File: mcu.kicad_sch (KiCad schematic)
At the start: 9 parts, among them SW1 Push_Button, SW2 Push_Button, U2 ESP32-S3-WROOM-1

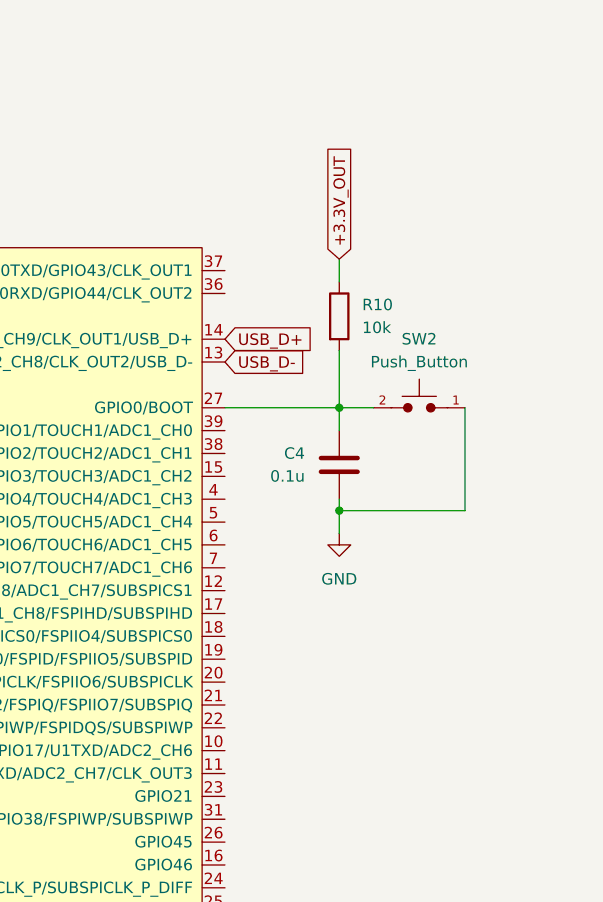
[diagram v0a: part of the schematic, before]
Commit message: Small ammendments
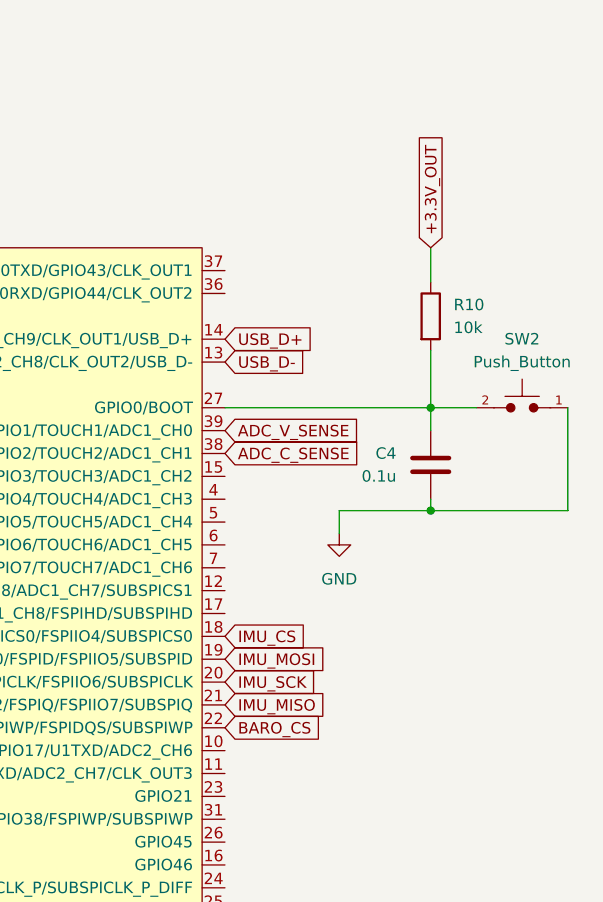
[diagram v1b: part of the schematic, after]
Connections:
- net IMU_CS: now reaches U2.18 (GPIO10/TOUCH10/ADC1_CH9/FSPICS0/FSPIIO4/SUBSPICS0)
- net IMU_MOSI: now reaches U2.19 (GPIO11/TOUCH11/ADC2_CH0/FSPID/FSPIIO5/SUBSPID)
- net IMU_SCK: now reaches U2.20 (GPIO12/TOUCH12/ADC2_CH1/FSPICLK/FSPIIO6/SUBSPICLK)
- net IMU_MISO: now reaches U2.21 (GPIO13/TOUCH13/ADC2_CH2/FSPIQ/FSPIIO7/SUBSPIQ)
- net BARO_CS: now reaches U2.22 (GPIO14/TOUCH14/ADC2_CH3/FSPIWP/FSPIDQS/SUBSPIWP)
- net ADC_C_SENSE: now reaches U2.38 (GPIO2/TOUCH2/ADC1_CH1)
- net ADC_V_SENSE: now reaches U2.39 (GPIO1/TOUCH1/ADC1_CH0)
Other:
- moved on the sheet: C4, R10, SW2
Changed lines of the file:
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@@
 	(paper "A4")
+	(junction
+		(at 156.21 67.31)
+		(diameter 0)
+		(color 0 0 0 0)
+	)
 	(junction
 		(at 76.2 25.4)
@@
 	)
 	(junction
-		(at 146.05 78.74)
+		(at 156.21 78.74)
 		(diameter 0)
 		(color 0 0 0 0)
@@
 	)
 	(junction
-		(at 146.05 67.31)
-		(diameter 0)
-		(color 0 0 0 0)
-	)
-	(junction
 		(at 68.58 36.83)
 		(diameter 0)
@@
 	(wire
 		(pts
+			(xy 146.05 78.74) (xy 146.05 81.28)
+		)
+		(stroke
+			(width 0)
+			(type default)
+		)
+	)
+	(wire
+		(pts
 			(xy 76.2 25.4) (xy 87.63 25.4)
 		)
@@
 	(wire
 		(pts
-			(xy 146.05 67.31) (xy 149.86 67.31)
+			(xy 156.21 67.31) (xy 161.29 67.31)
 		)
 		(stroke
@@
 	(wire
 		(pts
-			(xy 160.02 67.31) (xy 160.02 78.74)
+			(xy 171.45 67.31) (xy 171.45 78.74)
 		)
 		(stroke
@@
 	(wire
 		(pts
-			(xy 146.05 78.74) (xy 160.02 78.74)
+			(xy 146.05 78.74) (xy 156.21 78.74)
 		)
 		(stroke
@@
 	(wire
 		(pts
-			(xy 146.05 67.31) (xy 146.05 69.85)
+			(xy 156.21 67.31) (xy 156.21 69.85)
 		)
 		(stroke
@@
 	(wire
 		(pts
-			(xy 133.35 67.31) (xy 146.05 67.31)
+			(xy 133.35 67.31) (xy 156.21 67.31)
 		)
 		(stroke
@@
 	(wire
 		(pts
+			(xy 156.21 49.53) (xy 156.21 53.34)
+		)
+		(stroke
+			(width 0)
+			(type default)
+		)
+	)
+	(wire
+		(pts
 			(xy 33.02 49.53) (xy 33.02 54.61)
 		)
@@
 	(wire
 		(pts
-			(xy 146.05 50.8) (xy 146.05 53.34)
+			(xy 156.21 78.74) (xy 171.45 78.74)
 		)
 		(stroke
@@
 	(wire
 		(pts
-			(xy 146.05 60.96) (xy 146.05 67.31)
-		)
-		(stroke
-			(width 0)
-			(type default)
-		)
-	)
-	(wire
-		(pts
-			(xy 146.05 77.47) (xy 146.05 81.28)
-		)
-		(stroke
-			(width 0)
-			(type default)
+			(xy 156.21 60.96) (xy 156.21 67.31)
+		)
+		(stroke
+			(width 0)
+			(type default)
+		)
+	)
+	(wire
+		(pts
+			(xy 156.21 77.47) (xy 156.21 78.74)
+		)
+		(stroke
+			(width 0)
+			(type default)
+		)
+	)
+	(global_label "IMU_MOSI"
+		(shape input)
+		(at 133.35 95.25 0)
+		(fields_autoplaced yes)
+		(effects
+			(font
+				(size 1.27 1.27)
+			)
+			(justify left)
+		)
+		(property "Intersheetrefs" "${INTERSHEET_REFS}"
+			(at 145.2857 95.25 0)
+			(hide yes)
+			(show_name no)
+			(do_not_autoplace no)
+			(effects
+				(font
+					(size 1.27 1.27)
+				)
+				(justify left)
+			)
+		)
+	)
+	(global_label "IMU_CS"
+		(shape input)
+		(at 133.35 92.71 0)
+		(fields_autoplaced yes)
+		(effects
+			(font
+				(size 1.27 1.27)
+			)
+			(justify left)
+		)
+		(property "Intersheetrefs" "${INTERSHEET_REFS}"
+			(at 143.169 92.71 0)
+			(hide yes)
+			(show_name no)
+			(do_not_autoplace no)
+			(effects
+				(font
+					(size 1.27 1.27)
+				)
+				(justify left)
+			)
+		)
+	)
+	(global_label "ADC_C_SENSE"
+		(shape input)
+		(at 133.35 72.39 0)
+		(fields_autoplaced yes)
+		(effects
+			(font
+				(size 1.27 1.27)
+			)
+			(justify left)
+		)
+		(property "Intersheetrefs" "${INTERSHEET_REFS}"
+			(at 149.2165 72.39 0)
+			(hide yes)
+			(show_name no)
+			(do_not_autoplace no)
+			(effects
+				(font
+					(size 1.27 1.27)
+				)
+				(justify left)
+			)
 		)
 	)
@@
 		)
 	)
+	(global_label "BARO_CS"
+		(shape input)
+		(at 133.35 102.87 0)
+		(fields_autoplaced yes)
+		(effects
+			(font
+				(size 1.27 1.27)
+			)
+			(justify left)
+		)
+		(property "Intersheetrefs" "${INTERSHEET_REFS}"
+			(at 144.7414 102.87 0)
+			(hide yes)
+			(show_name no)
+			(do_not_autoplace no)
+			(effects
+				(font
+					(size 1.27 1.27)
+				)
+				(justify left)
+			)
+		)
+	)
+	(global_label "IMU_SCK"
+		(shape input)
+		(at 133.35 97.79 0)
+		(fields_autoplaced yes)
+		(effects
+			(font
+				(size 1.27 1.27)
+			)
+			(justify left)
+		)
+		(property "Intersheetrefs" "${INTERSHEET_REFS}"
+			(at 144.439 97.79 0)
+			(hide yes)
+			(show_name no)
+			(do_not_autoplace no)
+			(effects
+				(font
+					(size 1.27 1.27)
+				)
+				(justify left)
+			)
+		)
+	)
 	(global_label "+3.3V_OUT"
 		(shape input)
@@
 		)
 	)
-	(global_label "+3.3V_OUT"
+	(global_label "IMU_MISO"
 		(shape input)
-		(at 146.05 50.8 90)
+		(at 133.35 100.33 0)
 		(fields_autoplaced yes)
 		(effects
@@
 		)
 		(property "Intersheetrefs" "${INTERSHEET_REFS}"
-			(at 146.05 37.5338 90)
+			(at 145.2857 100.33 0)
+			(hide yes)
+			(show_name no)
+			(do_not_autoplace no)
+			(effects
+				(font
+					(size 1.27 1.27)
+				)
+				(justify left)
+			)
+		)
+	)
+	(global_label "+3.3V_OUT"
+		(shape input)
+		(at 156.21 49.53 90)
+		(fields_autoplaced yes)
+		(effects
+			(font
+				(size 1.27 1.27)
+			)
+			(justify left)
+		)
+		(property "Intersheetrefs" "${INTERSHEET_REFS}"
+			(at 156.21 36.2638 90)
+			(hide yes)
+			(show_name no)
+			(do_not_autoplace no)
+			(effects
+				(font
+					(size 1.27 1.27)
+				)
+				(justify left)
+			)
+		)
+	)
+	(global_label "ADC_V_SENSE"
+		(shape input)
+		(at 133.35 69.85 0)
+		(fields_autoplaced yes)
+		(effects
+			(font
+				(size 1.27 1.27)
+			)
+			(justify left)
+		)
+		(property "Intersheetrefs" "${INTERSHEET_REFS}"
+			(at 149.0351 69.85 0)
 			(hide yes)
 			(show_name no)
@@
 	(symbol
 		(lib_id "PCM_SL_Devices:Push_Button")
-		(at 154.94 67.31 0)
+		(at 166.37 67.31 0)
 		(mirror y)
 		(unit 1)
@@
 		(fields_autoplaced yes)
 		(property "Reference" "SW2"
-			(at 154.94 59.69 0)
+			(at 166.37 59.69 0)
 			(show_name no)
 			(do_not_autoplace no)
@@
 		)
 		(property "Value" "Push_Button"
-			(at 154.94 62.23 0)
+			(at 166.37 62.23 0)
 			(show_name no)
 			(do_not_autoplace no)
@@
 		)
 		(property "Footprint" "Button_Switch_THT:SW_PUSH_6mm"
-			(at 155.067 70.485 0)
+			(at 166.497 70.485 0)
 			(hide yes)
 			(show_name no)
@@
 		)
 		(property "Datasheet" ""
-			(at 154.94 67.31 0)
+			(at 166.37 67.31 0)
 			(hide yes)
 			(show_name no)
@@
 		)
 		(property "Description" "Common 6mmx6mm Push Button"
-			(at 154.94 67.31 0)
+			(at 166.37 67.31 0)
 			(hide yes)
 			(show_name no)
@@
 	(symbol
 		(lib_id "Device:C")
-		(at 146.05 73.66 0)
+		(at 156.21 73.66 0)
 		(mirror y)
 		(unit 1)
@@
 		(fields_autoplaced yes)
 		(property "Reference" "C4"
-			(at 142.24 72.3899 0)
+			(at 152.4 72.3899 0)
 			(show_name no)
 			(do_not_autoplace no)
@@
 		)
 		(property "Value" "0.1u"
-			(at 142.24 74.9299 0)
+			(at 152.4 74.9299 0)
 			(show_name no)
 			(do_not_autoplace no)
@@
 		)
 		(property "Footprint" ""
-			(at 145.0848 77.47 0)
+			(at 155.2448 77.47 0)
 			(hide yes)
 			(show_name no)
@@
 		)
 		(property "Datasheet" ""
-			(at 146.05 73.66 0)
+			(at 156.21 73.66 0)
 			(hide yes)
 			(show_name no)
@@
 		)
 		(property "Description" "Unpolarized capacitor"
-			(at 146.05 73.66 0)
+			(at 156.21 73.66 0)
 			(hide yes)
 			(show_name no)
@@
 	(symbol
 		(lib_id "Device:R")
-		(at 146.05 57.15 0)
+		(at 156.21 57.15 0)
 		(unit 1)
 		(body_style 1)
@@
 		(fields_autoplaced yes)
 		(property "Reference" "R10"
-			(at 148.59 55.8799 0)
+			(at 158.75 55.8799 0)
 			(show_name no)
 			(do_not_autoplace no)
@@
 		)
 		(property "Value" "10k"
-			(at 148.59 58.4199 0)
+			(at 158.75 58.4199 0)
 			(show_name no)
 			(do_not_autoplace no)
@@
 		)
 		(property "Footprint" ""
-			(at 144.272 57.15 90)
+			(at 154.432 57.15 90)
 			(hide yes)
 			(show_name no)
@@
 		)
 		(property "Datasheet" ""
-			(at 146.05 57.15 0)
+			(at 156.21 57.15 0)
 			(hide yes)
 			(show_name no)
@@
 		)
 		(property "Description" "Resistor"
-			(at 146.05 57.15 0)
-			(hide yes)
-			(show_name no)
+			(at 156.21 57.15 0)
+			(hide yes)
+			(show_name no)

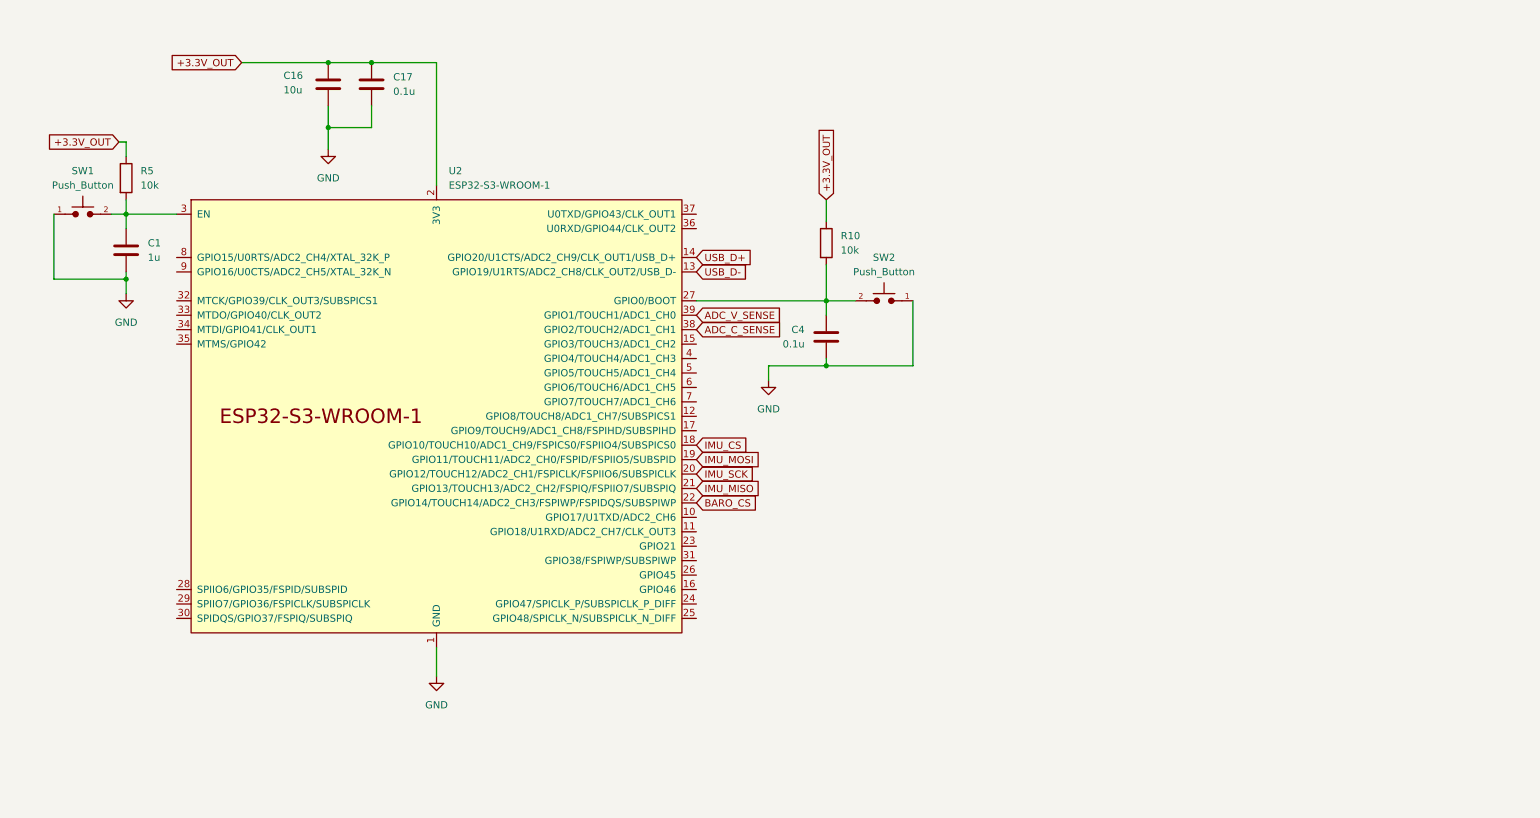
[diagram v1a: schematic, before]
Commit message: 8.09.2026 - 19:33
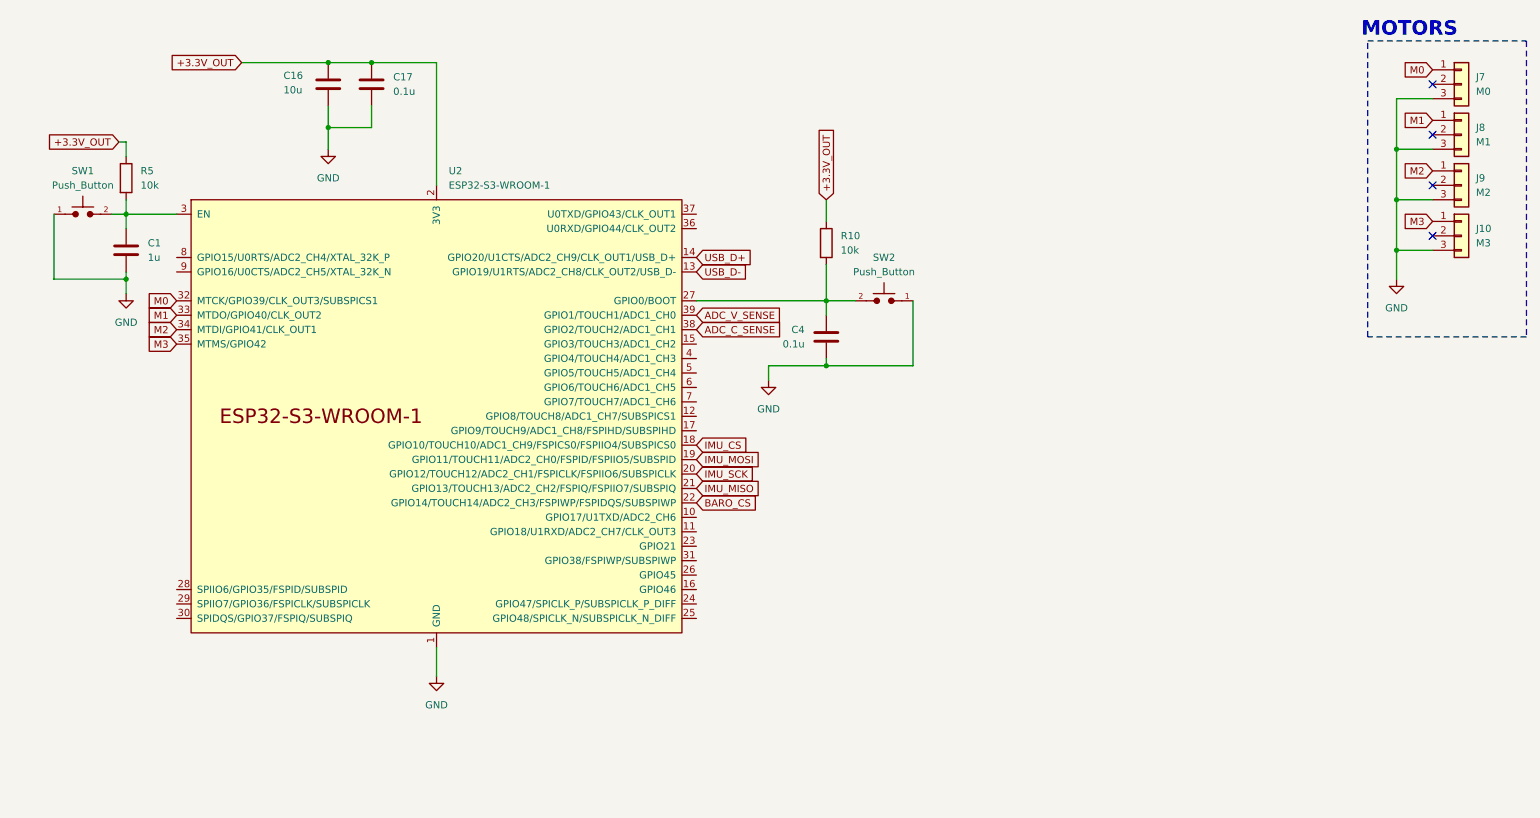
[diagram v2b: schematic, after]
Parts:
- added J10: M3, Connector_PinHeader_2.54mm:PinHeader_1x03_P2.54mm_Horizontal, symbol Connector_Generic:Conn_01x03
- added J7: M0, Connector_PinHeader_2.54mm:PinHeader_1x03_P2.54mm_Horizontal, symbol Connector_Generic:Conn_01x03
- added J8: M1, Connector_PinHeader_2.54mm:PinHeader_1x03_P2.54mm_Horizontal, symbol Connector_Generic:Conn_01x03
- added J9: M2, Connector_PinHeader_2.54mm:PinHeader_1x03_P2.54mm_Horizontal, symbol Connector_Generic:Conn_01x03
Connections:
- net GND: now also J10.3 (Pin_3), J7.3 (Pin_3), J8.3 (Pin_3), J9.3 (Pin_3)
- net M0: now reaches U2.32 (MTCK/GPIO39/CLK_OUT3/SUBSPICS1)
- net M0: now also J7.1 (Pin_1)
- net M1: now reaches U2.33 (MTDO/GPIO40/CLK_OUT2)
- net M1: now also J8.1 (Pin_1)
- net M2: now reaches U2.34 (MTDI/GPIO41/CLK_OUT1)
- net M2: now also J9.1 (Pin_1)
- net M3: now reaches U2.35 (MTMS/GPIO42)
- net M3: now also J10.1 (Pin_1)
- no-connect marks 0 -> 4
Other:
- note added: "MOTORS"

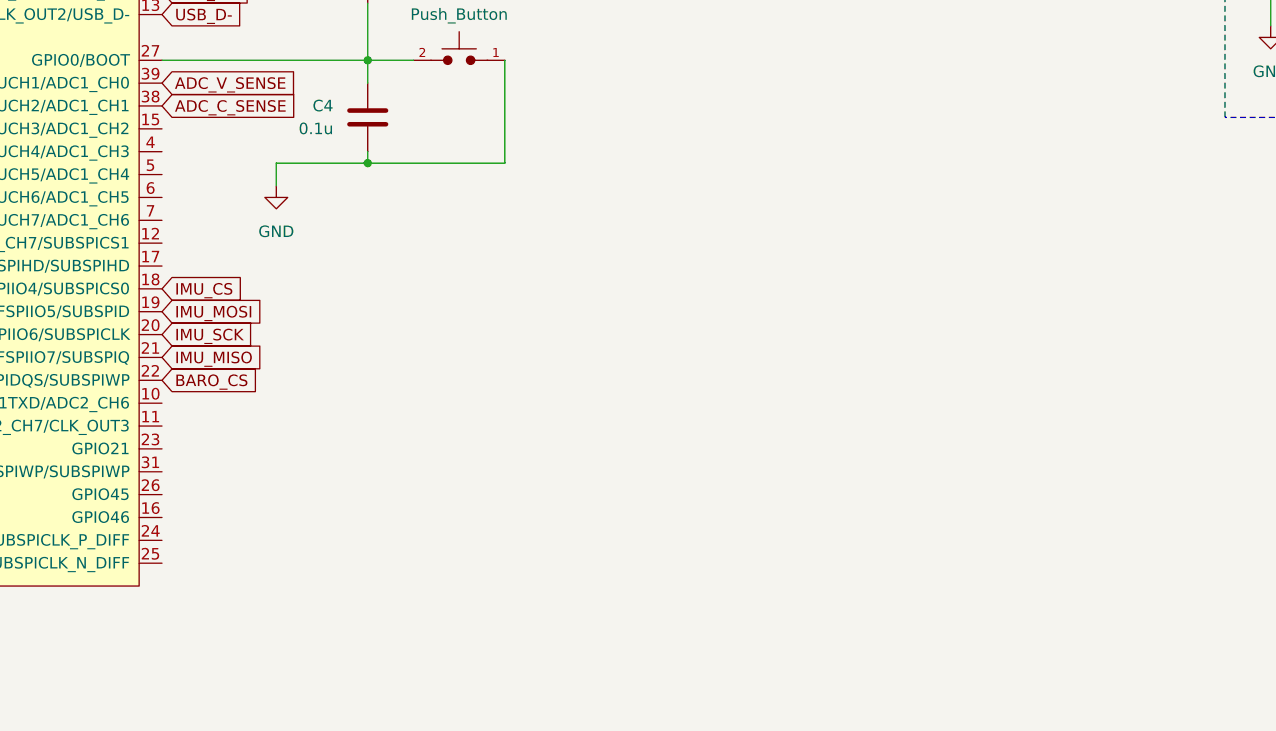
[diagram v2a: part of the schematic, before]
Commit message: 8.09.2026 - 20:26
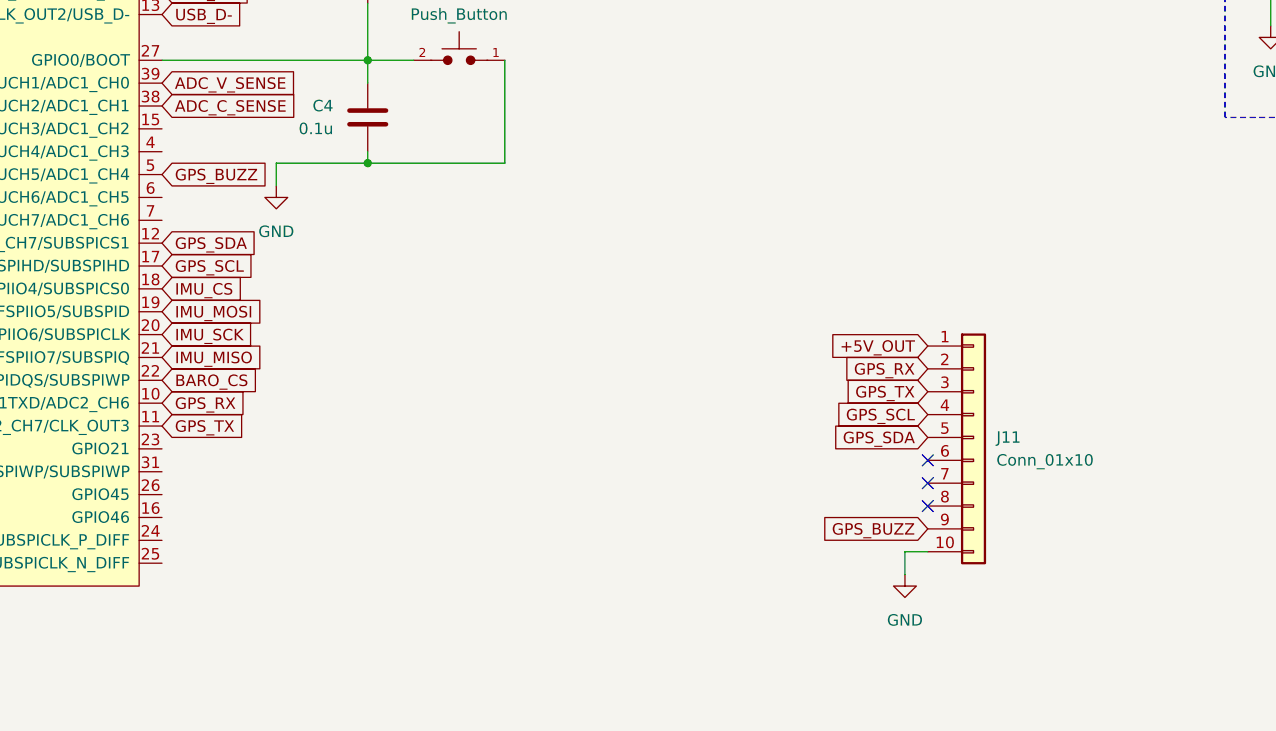
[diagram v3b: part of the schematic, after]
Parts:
- added J11: Conn_01x10, Connector_JST:JST_GH_BM10B-GHS-TBT_1x10-1MP_P1.25mm_Vertical, symbol Connector_Generic:Conn_01x10
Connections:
- net GND: now also J11.10 (Pin_10)
- net GPS_RX: now reaches U2.10 (GPIO17/U1TXD/ADC2_CH6)
- net GPS_RX: now also J11.2 (Pin_2)
- net GPS_TX: now reaches U2.11 (GPIO18/U1RXD/ADC2_CH7/CLK_OUT3)
- net GPS_TX: now also J11.3 (Pin_3)
- net GPS_SDA: now reaches U2.12 (GPIO8/TOUCH8/ADC1_CH7/SUBSPICS1)
- net GPS_SDA: now also J11.5 (Pin_5)
- net GPS_SCL: now reaches U2.17 (GPIO9/TOUCH9/ADC1_CH8/FSPIHD/SUBSPIHD)
- net GPS_SCL: now also J11.4 (Pin_4)
- net GPS_BUZZ: now reaches U2.5 (GPIO5/TOUCH5/ADC1_CH4)
- net GPS_BUZZ: now also J11.9 (Pin_9)
- new net +5V_OUT: J11.1 (Pin_1)
- no-connect marks 4 -> 7
